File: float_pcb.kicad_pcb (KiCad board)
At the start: 4 copper layers, 64 x 64 mm, 77 parts, among them J1 Switch, J2 Conn_01x04, J3 USB_C, J4 Conn_01x03, J5 I2C, J6 Light, J7 Batt, J9 I2C, Q1 AO3400A, Q2 AO3400A, U1 TPSM863252, U2 TPSM863252, U3 USBLC6-2SC6, U4 ESP32-S3-WROOM-1U, U5 USBLC6-4SC6, U6 USBLC6-4SC6

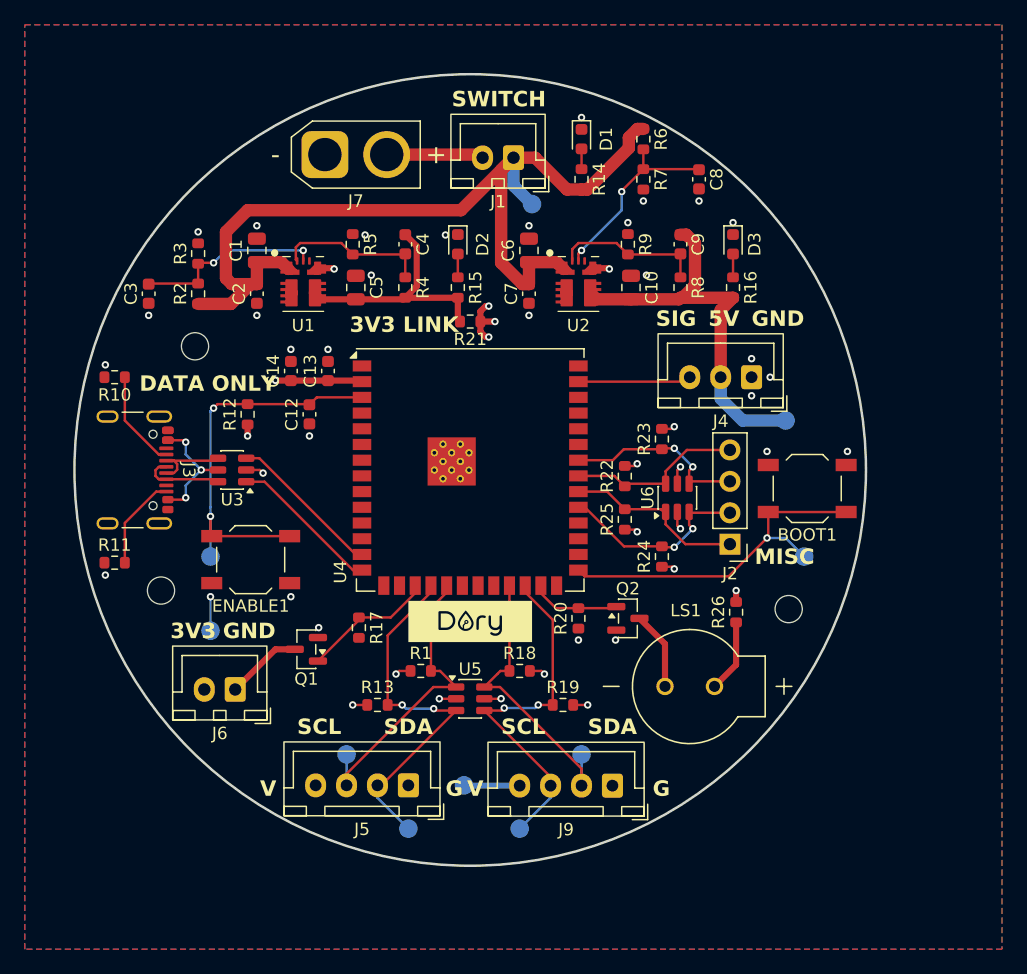
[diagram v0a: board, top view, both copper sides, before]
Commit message: V4
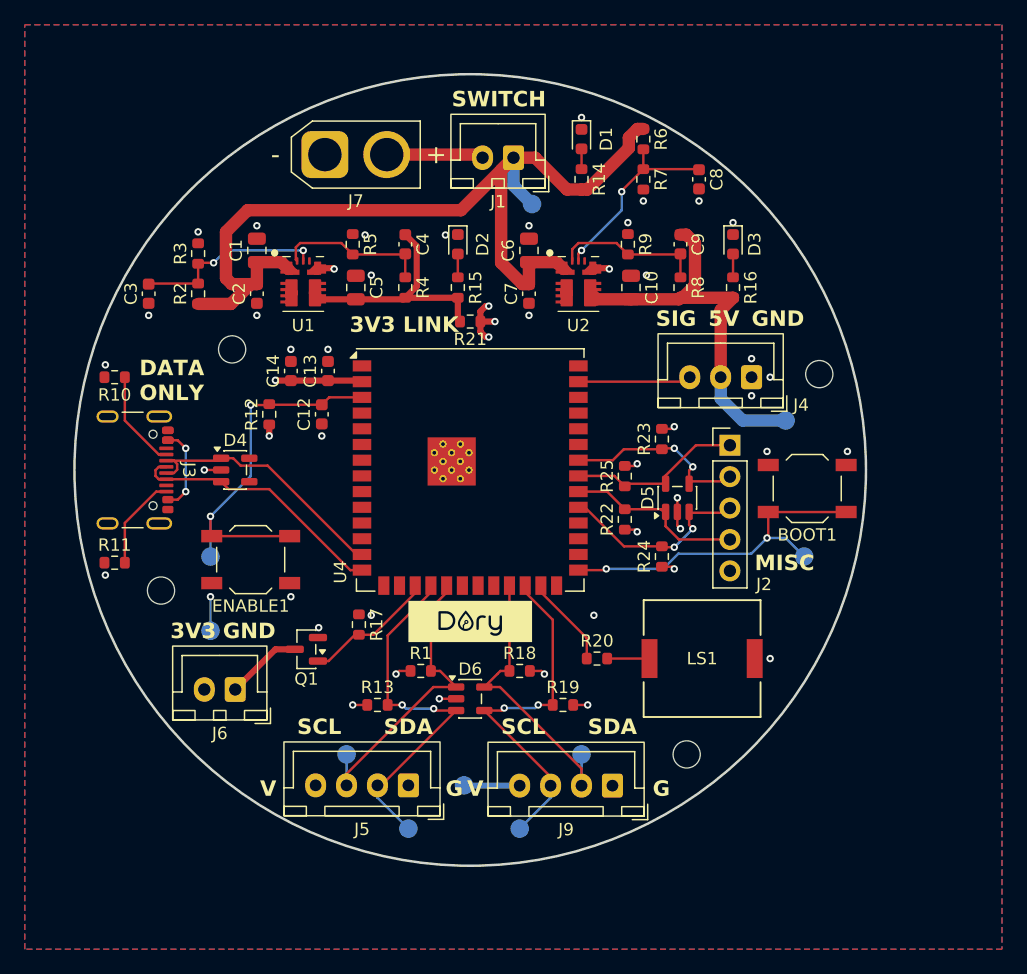
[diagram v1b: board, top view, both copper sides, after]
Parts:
- removed Q2: AO3400A, Package_TO_SOT_SMD:SOT-23
- removed R26: TBD, Resistor_SMD:R_0603_1608Metric
- removed U3: USBLC6-2SC6, Package_TO_SOT_SMD:SOT-23-6
- removed U5, U6: USBLC6-4SC6, Package_TO_SOT_SMD:SOT-23-6
- added D4: ESDS314, Package_TO_SOT_SMD:SOT-23-5, F.Cu at (129.5, 105.0)
- added D5: ESDS314, Package_TO_SOT_SMD:SOT-23-5, F.Cu at (165.2, 107.2)
- added D6: ESDS314, Package_TO_SOT_SMD:SOT-23-5, F.Cu at (148.5, 123.5)
- added H4: MH, MountingHole:MountingHole_2.2mm_M2, F.Cu at (176.7, 97.2)
- J2: value Conn_01x04 -> Conn_01x05; footprint Connector_PinHeader_2.54mm:PinHeader_1x04_P2.54mm_Vertical -> Connector_PinHeader_2.54mm:PinHeader_1x05_P2.54mm_Vertical
- LS1: value AT-1127-ST-2-R -> CPT-9019A-SMT-TR; footprint buzzer:XDCR_AT-1127-ST-2-R -> buzzer:CPT-9019A_CUD
- R20: value 10k -> 1k
- TP7: value SDA2 -> SDA1
- moved H2 14.4 mm to (166.0, 128.0)
- moved J2 8.00 mm to (169.5, 103.0), turned to 0 degrees
- moved R20 3.58 mm to (158.8, 120.2), turned to 0 degrees
- moved H1 3.01 mm to (129.2, 95.2)
- moved LS1 2.46 mm to (167.2, 120.2)
- moved R12 1.75 mm to (132.2, 100.5)
- moved C12 1.00 mm to (136.5, 100.5)
- moved R17 0.25 mm to (139.5, 117.5)
- renumbered R25 to R22, R22 to R25
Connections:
- net VBUS_USB renamed /USB_VBUS
- R17 pad 1: LIGHT -> GND
- R17 pad 2: GND -> LIGHT
- R20 pad 1: GND -> BUZZER
- R20 pad 2: BUZZER -> Net-(LS1-Pad1)
- R22 pad 2: MISC1 -> MISC4
- R23 pad 1: MISC3 -> MISC2
- R24 pad 2: MISC2 -> MISC3
- R25 pad 1: MISC4 -> MISC1
- U4 pad 13: ESP32_D- -> USBC_D-
- U4 pad 14: ESP32_D+ -> USBC_D+
- U4 pad 31: MISC2 -> MISC3
- U4 pad 32: MISC1 -> MISC4
- U4 pad 33: MISC4 -> MISC1
- U4 pad 34: MISC3 -> MISC2
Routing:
- net USBC_D-: track 6.70 -> 21.6 mm
- net USBC_D+: track 6.70 -> 21.3 mm
- net ESP32_D-: track 12.6 -> 0.00 mm
- net ESP32_D+: track 12.3 -> 0.00 mm
- net Net-(Q2-D): track 6.35 -> 0.00 mm
- net Net-(LS1-PadP): track 5.90 -> 0.00 mm
- net +3V3: track 30.0 -> 26.2 mm, vias 16 -> 13
- net Net-(LS1-Pad1): track 0.00 -> 3.42 mm
- net /USB_VBUS: track 9.92 -> 6.93 mm, vias 3 -> 2
- net Net-(U4-EN): track 32.4 -> 30.8 mm
- net MISC3: track 14.9 -> 16.0 mm
- net MISC2: track 16.0 -> 14.9 mm
- net GND: track 9.77 -> 10.8 mm, vias 35 -> 37
- net Net-(U4-IO0): track 28.8 -> 28.4 mm, vias 1 -> 2
